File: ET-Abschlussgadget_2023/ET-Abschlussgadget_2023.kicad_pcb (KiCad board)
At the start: 2 copper layers, 85 x 54 mm, 0 parts

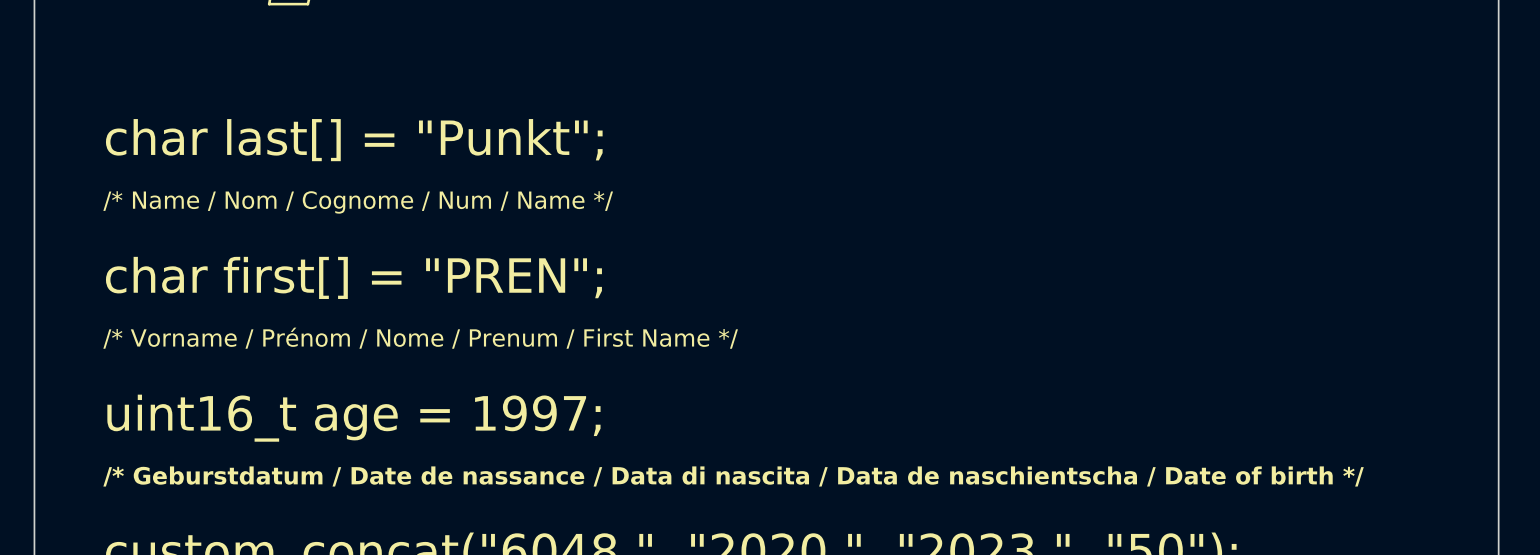
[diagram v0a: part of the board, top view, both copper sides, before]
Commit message: Added first & last name
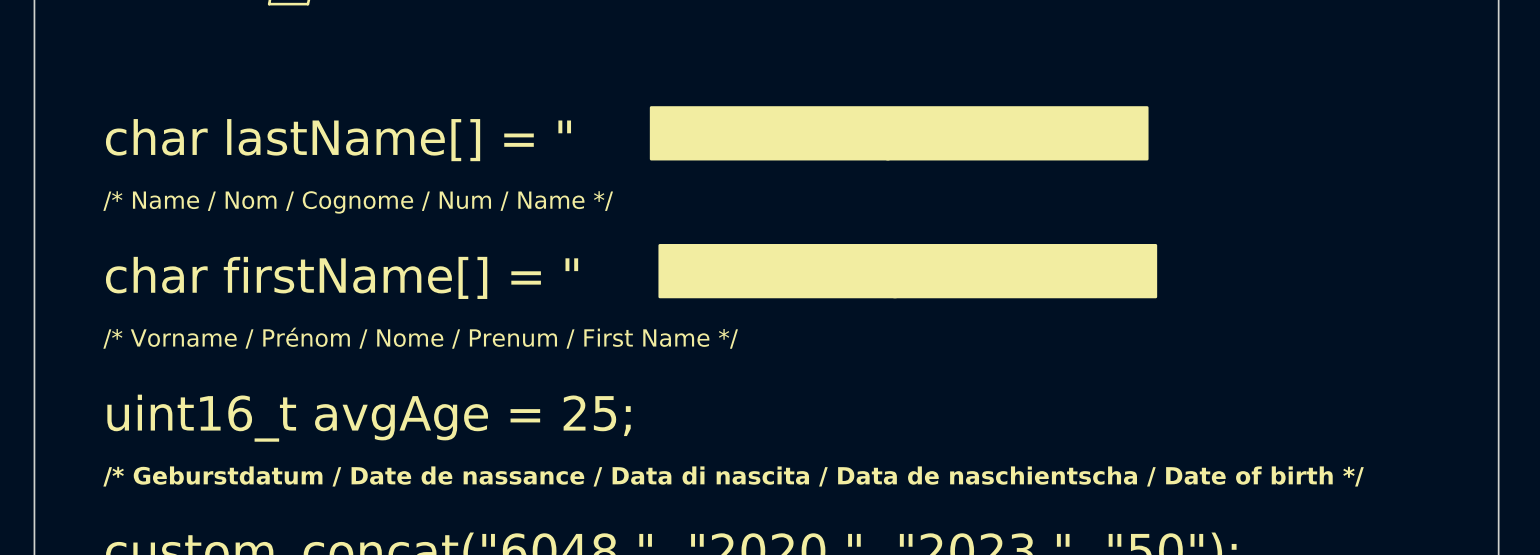
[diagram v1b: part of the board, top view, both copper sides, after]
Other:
- board text added: "char firstName[] = {dblquote} {dblquote};"
- board text added: "char lastName[] = {dblquote} {dblquote};"
- board text added: "uint16_t avgAge = 25;"
- board text removed: "char first[] = {dblquote}PREN{dblquote};"
- board text removed: "char last[] = {dblquote}Punkt{dblquote};"
- board text removed: "uint16_t age = 1997;"
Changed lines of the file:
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@@
   (gr_line (start 113.625 95) (end 115.875 95)
     (stroke (width 0.15) (type default)) (layer "F.SilkS"))
+  (gr_poly
+    (pts
+      (xy 136.3 109)
+      (xy 165.1 109)
+      (xy 165.1 112)
+      (xy 136.3 112)
+    )
+    (stroke (width 0.15) (type solid)) (fill solid) (layer "F.SilkS"))
+  (gr_poly
+    (pts
+      (xy 135.8 101)
+      (xy 164.6 101)
+      (xy 164.6 104)
+      (xy 135.8 104)
+    )
+    (stroke (width 0.15) (type solid)) (fill solid) (layer "F.SilkS"))
   (gr_line (start 116.175 88.525) (end 114.925 88.525)
     (stroke (width 0.15) (type default)) (layer "F.SilkS"))
@@
     )
   )
-  (gr_text "uint16_t age = 1997;" (at 104 120) (layer "F.SilkS")
+  (gr_text "uint16_t avgAge = 25;" (at 104 120) (layer "F.SilkS")
     (effects (font (size 2 2) (thickness 0.3)) (justify left bottom))
   )
-  (gr_text "char last[] = {dblquote}Punkt{dblquote};" (at 104 104) (layer "F.SilkS")
+  (gr_text "char lastName[] = {dblquote}                   {dblquote};" (at 104 104) (layer "F.SilkS")
     (effects (font (size 2 2) (thickness 0.3)) (justify left bottom))
   )
@@
     (effects (font (size 1 1) (thickness 0.2) bold) (justify left bottom))
   )
-  (gr_text "char first[] = {dblquote}PREN{dblquote};" (at 104 112) (layer "F.SilkS")
+  (gr_text "char firstName[] = {dblquote}                   {dblquote};" (at 104 112) (layer "F.SilkS")
     (effects (font (size 2 2) (thickness 0.3)) (justify left bottom))
   )
